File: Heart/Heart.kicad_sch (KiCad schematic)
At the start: 22 parts, among them SW1 EG1218, SW2 BLINKY, U1 ATtiny85-20PU

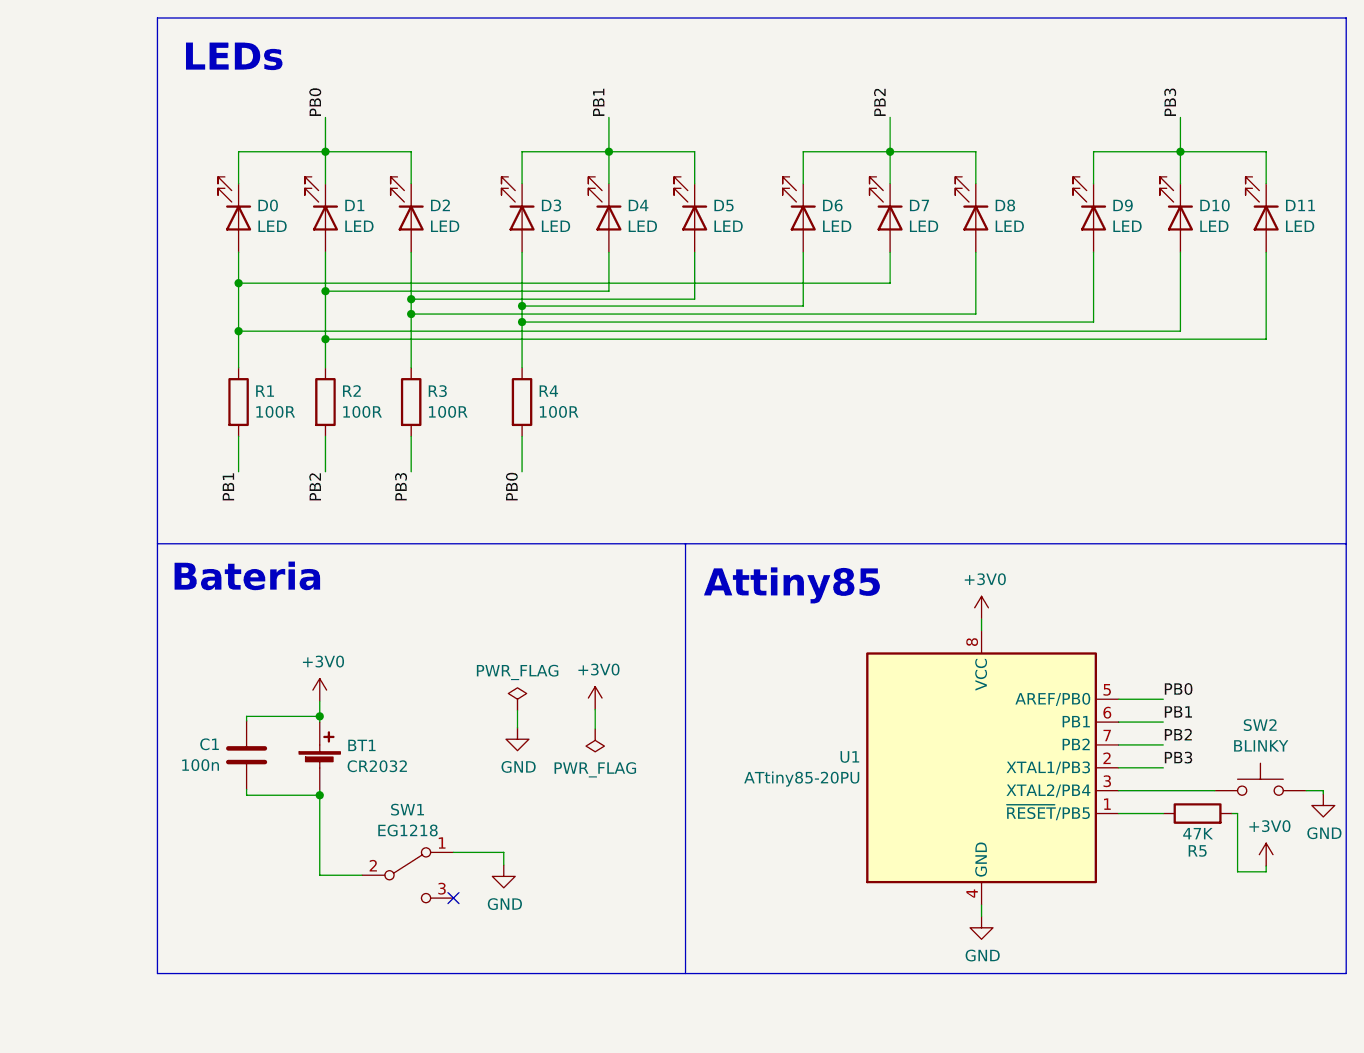
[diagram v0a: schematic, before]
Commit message: update files
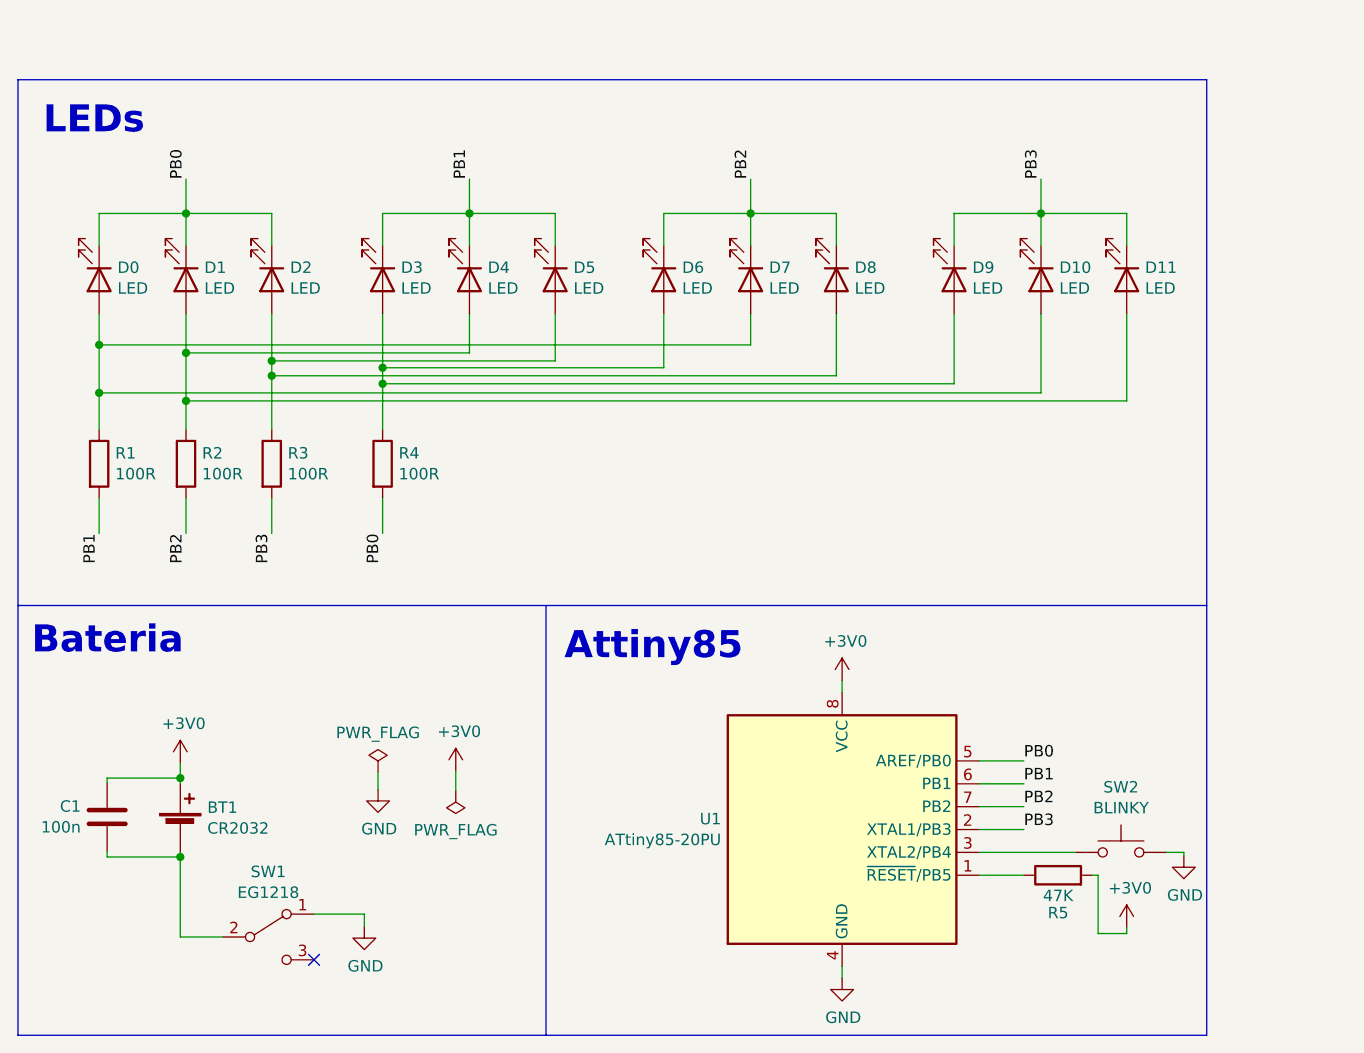
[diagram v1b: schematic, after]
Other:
- company: (none) -> Cristóbal Cuevas Lagos
- title: (none) -> Heart
- moved on the sheet: BT1, C1, D0, D1, D10, D11, D2, D3, D4, D5, D6, D7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
